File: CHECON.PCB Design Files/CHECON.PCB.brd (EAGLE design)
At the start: 81.7 x 51.7 mm, 72 parts

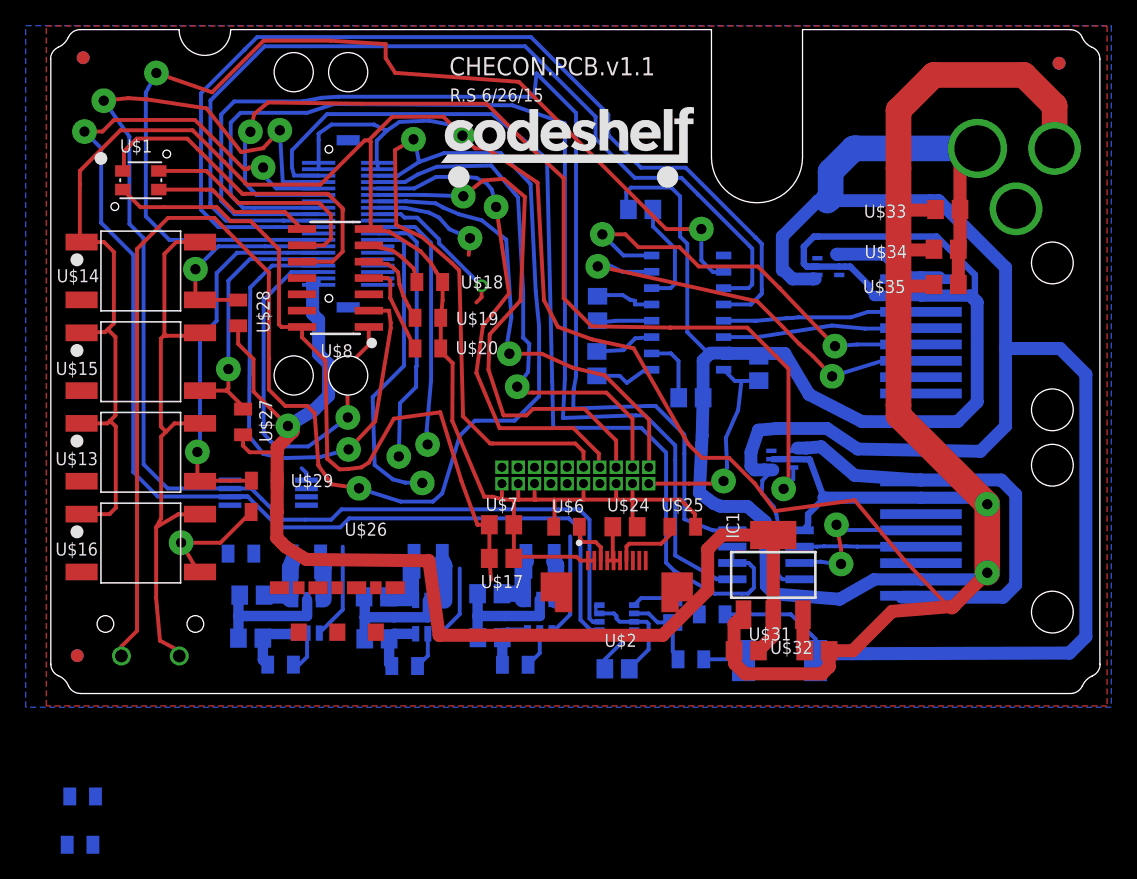
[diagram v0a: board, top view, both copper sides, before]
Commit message: Finished layout pending spring connector
Waiting for physical location of BL connector
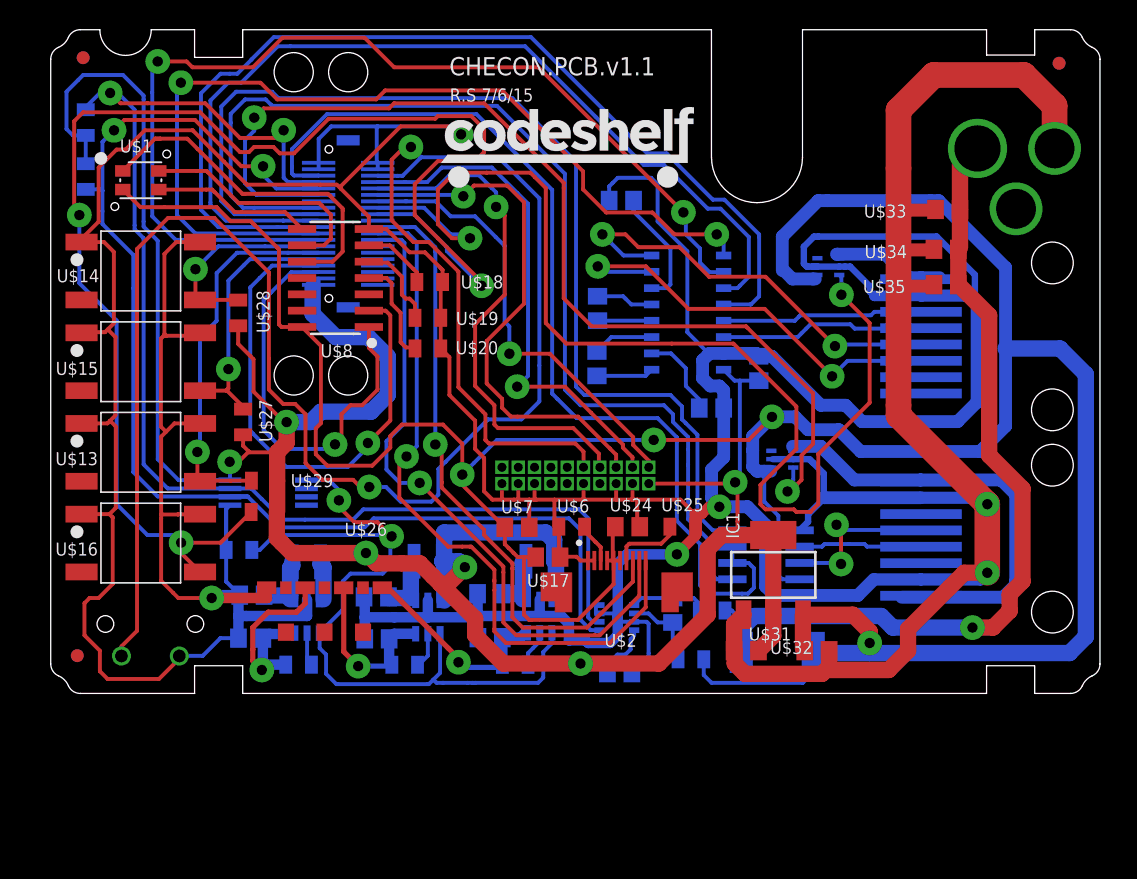
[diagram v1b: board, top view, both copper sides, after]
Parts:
- U$56: value 6.6 -> 6.8
- U$62: device texas:DCN-R-PDSO-G8 -> KW2:DCN-R-PDSO-G8
- moved U$61 52.4 mm to (-38.1, 18.6), turned to 90 degrees
- moved U$60 52.0 mm to (-38.1, 14.4), turned to 270 degrees
- moved U$17 3.60 mm to (-2.14, -15.2)
- moved U$22 1.79 mm to (10.6, -3.62)
- moved U$23 1.66 mm to (3.58, 12.5)
- moved U$58 1.40 mm to (-21.5, -23.6)
- moved U$7 1.22 mm to (-4.54, -12.9)
- moved U$59 1.00 mm to (-19.5, -17.6)
- moved R10 0.66 mm to (15.7, -22.6), turned to 180 degrees
- moved U$6 0.40 mm to (-0.29, -12.9)
- moved C14 0.36 mm to (3.45, -24.2)
- moved U$46 0.32 mm to (-26.2, -14.7), turned to 180 degrees
- moved R12 0.30 mm to (10.6, -19.4)
- moved U$24 0.20 mm to (4.06, -12.9)
- moved U$57 0.10 mm to (-13.3, -23.6)
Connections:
- removed net N$58: IC1.3, R10.2, R13.2, U$31.2
- new net N$49: R10.1, R12.2, U$33.2, U$34.2, U$35.2, U$9.P$1
- net GND: now also U$2.P$1, U$2.P$2; no longer U$2.P$10, U$2.P$9
- net N$29: now also U$2.P$9; no longer U$2.P$2
- net N$30: now also U$2.P$10; no longer U$2.P$1
- net N$31: now also U$2.P$8; no longer U$2.P$3
- net N$32: now also U$2.P$3; no longer U$2.P$8
- net N$33: now also U$2.P$7; no longer U$2.P$4
- net V+: now also IC1.3, R10.2, R13.2, U$2.P$4, U$31.2; no longer R10.1, R12.2, U$2.P$7, U$33.2, U$34.2, U$35.2, U$9.P$1
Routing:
- net N$42: track 22.2 -> 112.1 mm, vias 2 -> 3
- net +3V3: track 127.0 -> 216.7 mm, vias 2 -> 6
- net N$40: track 9.16 -> 90.2 mm, vias 1 -> 2
- net N$38: track 0.00 -> 71.9 mm, vias 0 -> 2
- net N$49: track 0.00 -> 67.0 mm, vias 0 -> 1
- net N$43: track 22.4 -> 60.6 mm, vias 0 -> 2
- net N$30: track 20.5 -> 55.2 mm
- net V+: track 222.9 -> 252.5 mm, vias 0 -> 4
- net N$31: track 20.4 -> 49.2 mm
- net N$29: track 24.6 -> 52.0 mm
- net N$54: track 4.61 -> 16.6 mm, vias 0 -> 1
- net N$51: track 5.46 -> 17.1 mm, vias 0 -> 1
- net N$53: track 4.43 -> 13.6 mm, vias 0 -> 1
- net N$58: track 6.00 -> 0.00 mm
- net GND: track 550.5 -> 555.1 mm, vias 3 -> 6
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- removed copper zone on layer 1, net GND
- removed copper zone on layer 16, net GND
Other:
- board size 81.7 x 51.7 mm -> 81.7 x 51.6 mm
- board text added: "R.S 7/6/15"
- board text removed: "R.S 6/26/15"
